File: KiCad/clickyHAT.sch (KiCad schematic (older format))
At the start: 16 parts, among them J1 Raspberry_Pi_2_3, Q1 BS170, SW1 SW_Push, SW2 SW_Push, SW3 SW_Push, SW4 SW_Push

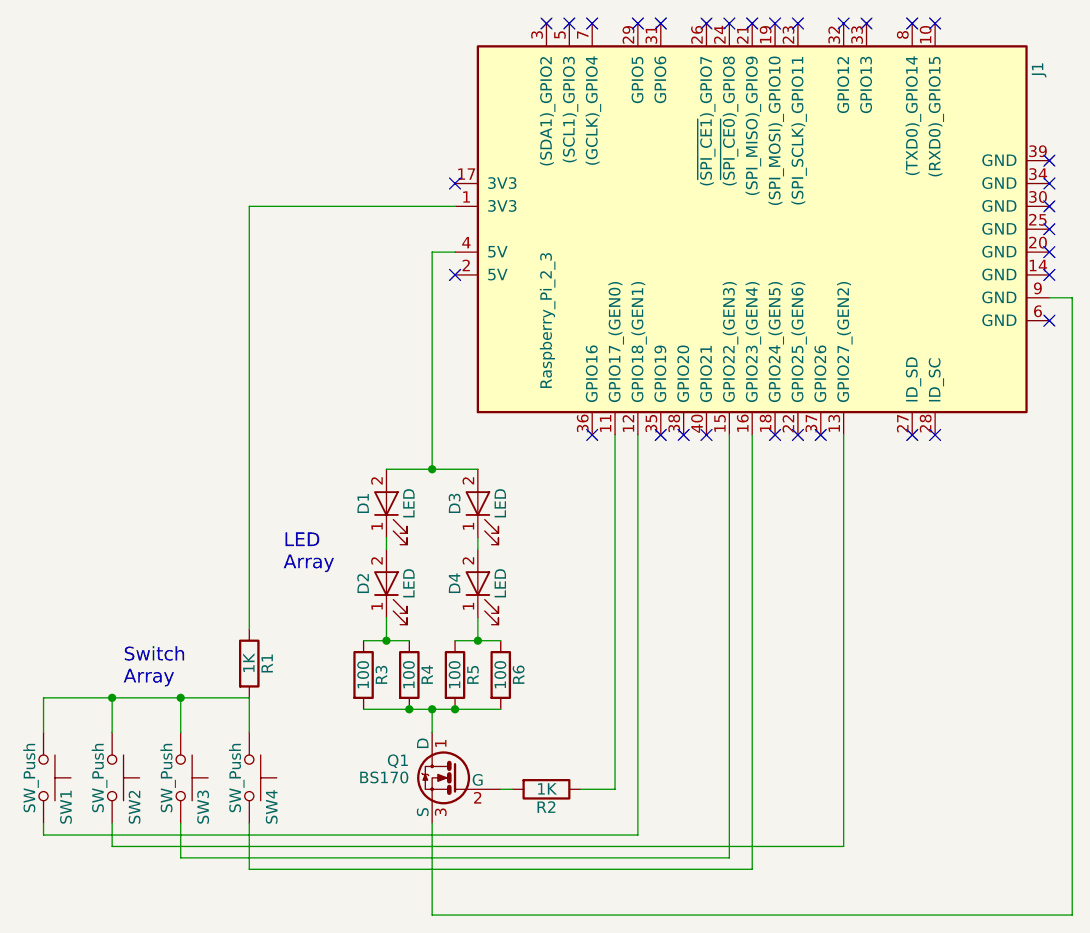
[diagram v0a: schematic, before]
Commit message: Revision 1.1
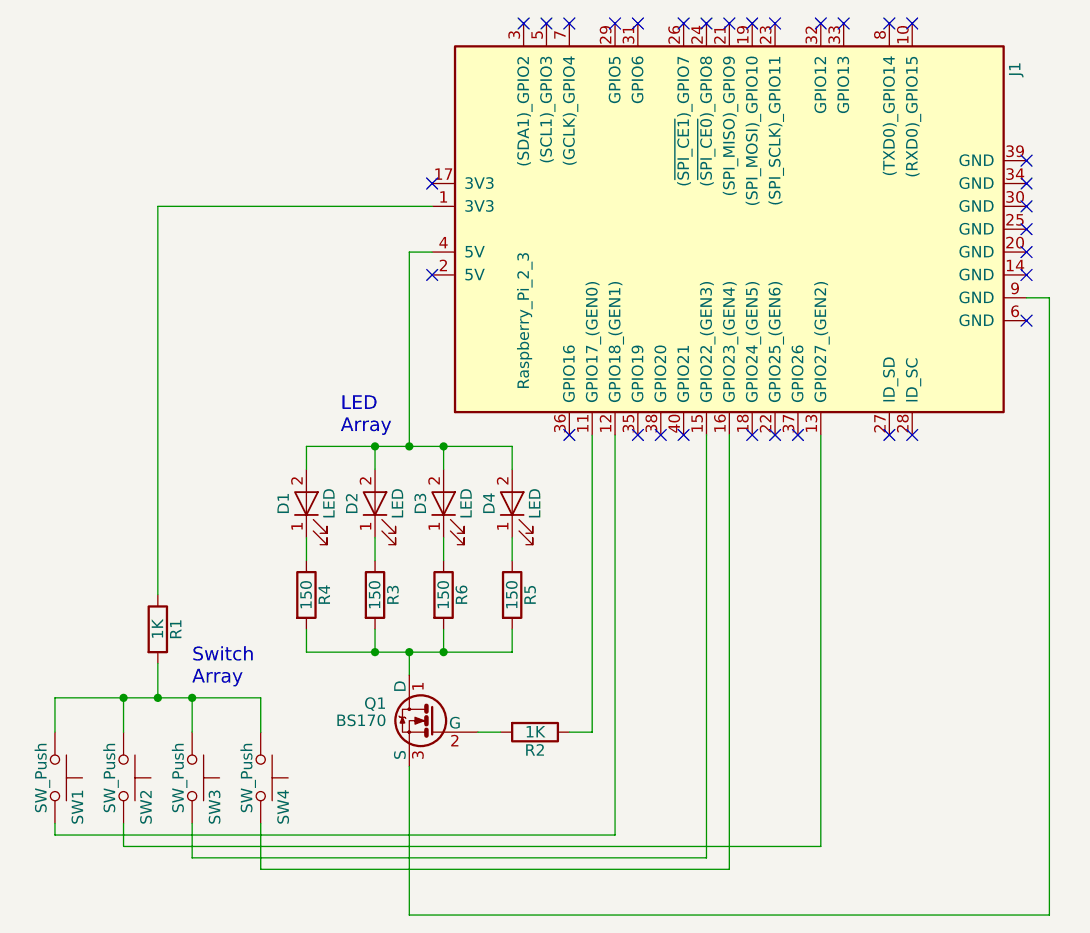
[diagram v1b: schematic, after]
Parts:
- R3: renamed from R4; value 100 -> 150
- R4: renamed from R3; value 100 -> 150
- R5: renamed from R6; value 100 -> 150
- R6: renamed from R5; value 100 -> 150
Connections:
- net at D1.2 (A), D3.2 (A), J1.4 (5V): now also D2.2 (A), D4.2 (A)
- net at D1.1 (K): now also R4.1; no longer D2.2 (A)
- net at D2.1 (K), R3.1: no longer R4.1
- net at D3.1 (K): now also R6.1; no longer D4.2 (A)
- net at D4.1 (K), R5.1: no longer R6.1
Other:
- moved on the sheet: D1, D2, D3, D4, J1, Q1, R1, R2, R3, R4, R5, R6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
